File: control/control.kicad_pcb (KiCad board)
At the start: 2 copper layers, 39.1 x 45.8 mm, 37 parts, among them J1 AVR-ISP-6, J2 Conn_01x07_Pin, J3 Conn_01x02_Pin, J4 Conn_01x04_Socket, P1 Conn_01x03_Pin, P2 Conn_01x03_Pin, P3 Conn_01x03_Pin, P4 Conn_01x03_Pin, SW1 SW_Push, U2 ATmega328P-A, Y1 16MHz

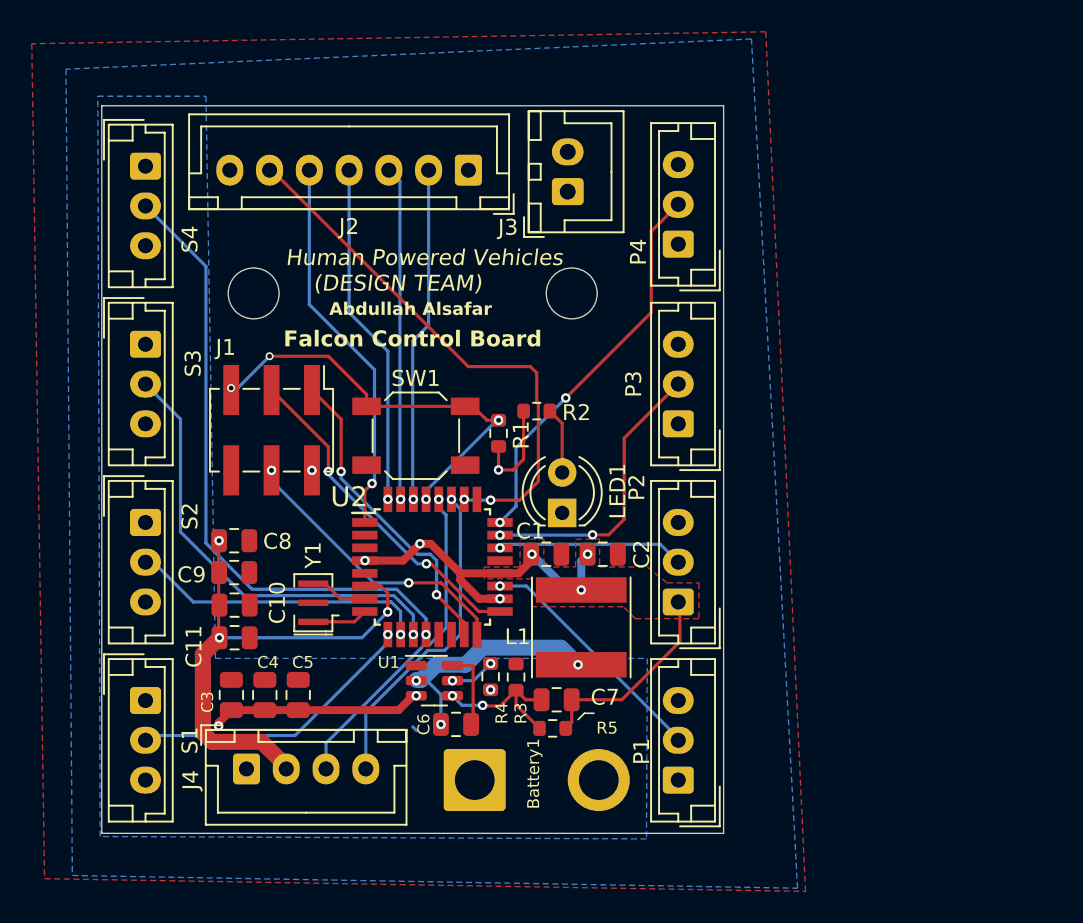
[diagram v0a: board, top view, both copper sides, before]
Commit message: Revised hardware
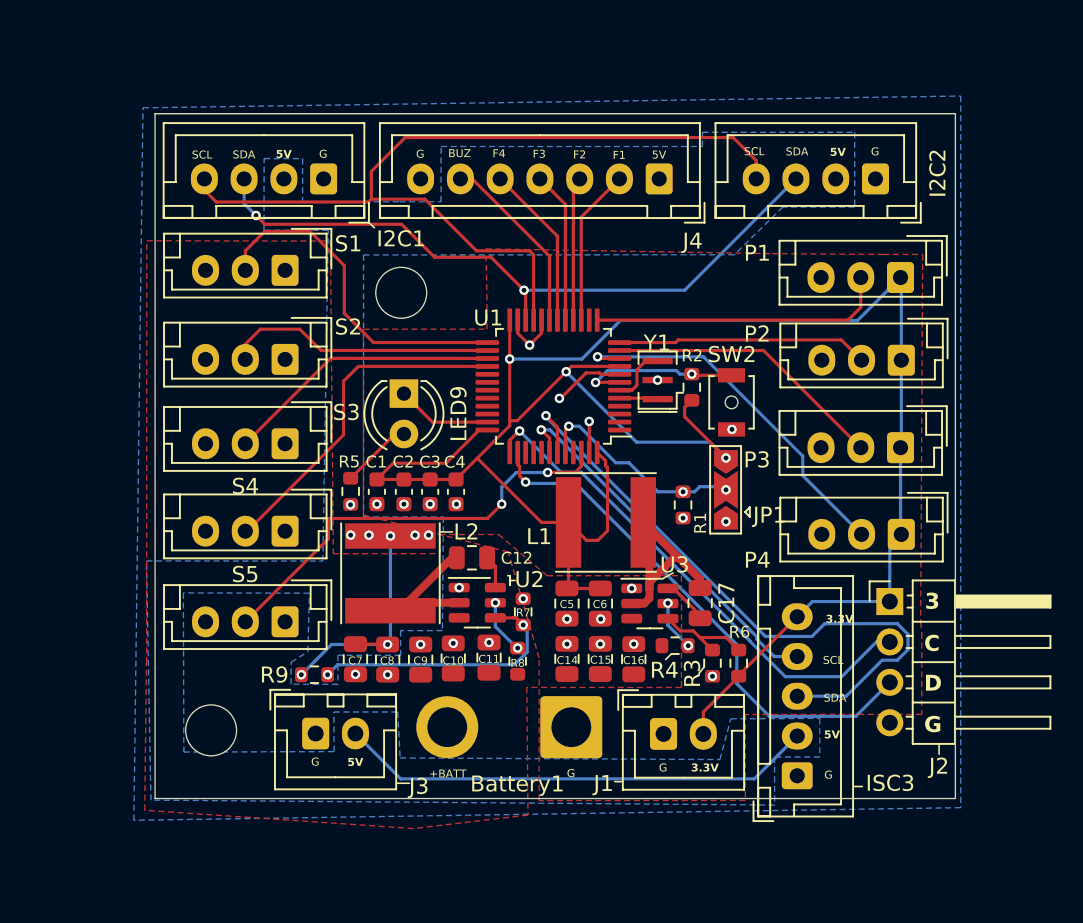
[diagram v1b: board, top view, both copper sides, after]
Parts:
- removed HOLE1, HOLE2: MountingHole_3.2mm_M3, MountingHole:MountingHole_3.2mm_M3
- removed LED1: LED1, LED_THT:LED_D4.0mm
- removed SW1: SW_Push, Button_Switch_SMD:SW_SPST_SKQG_WithoutStem
- added C12: 0.1uF, Capacitor_SMD:C_0805_2012Metric, F.Cu at (135.7, 84.4)
- added C14: 22uF, Capacitor_SMD:C_0805_2012Metric, F.Cu at (141.7, 90.8)
- added C15: 22uF, Capacitor_SMD:C_0805_2012Metric, F.Cu at (143.8, 90.8)
- added C16: 22uF, Capacitor_SMD:C_0805_2012Metric, F.Cu at (145.9, 90.8)
- added C17: 0.1uF, Capacitor_SMD:C_0805_2012Metric, F.Cu at (150.1, 87.3)
- added I2C1: FS2, Connector_JST:JST_XH_B4B-XH-A_1x04_P2.50mm_Vertical, F.Cu at (126.4, 60.6)
- added I2C2: FS1, Connector_JST:JST_XH_B4B-XH-A_1x04_P2.50mm_Vertical, F.Cu at (161.1, 60.6)
- added ISC3: MAIN, Connector_JST:JST_XH_B5B-XH-A_1x05_P2.50mm_Vertical, F.Cu at (156.2, 98.1)
- added JP1: Jumper_3_Open, Jumper:SolderJumper-3_P2.0mm_Open_TrianglePad1.0x1.5mm, F.Cu at (151.7, 80.2)
- added L2: 3.3uH, Inductor_SMD:L_Taiyo-Yuden_NR-60xx, F.Cu at (130.6, 85.4)
- added LED9: LED1, LED_THT:LED_D4.0mm, F.Cu at (131.4, 74.1)
- added R6: 33.2k, Resistor_SMD:R_0603_1608Metric, F.Cu at (152.5, 91.0)
- added R7: 10k, Resistor_SMD:R_0603_1608Metric, F.Cu at (138.9, 87.8)
- added R8: 10k, Resistor_SMD:R_0603_1608Metric, F.Cu at (138.6, 90.9)
- added R9: 54.9k, Resistor_SMD:R_0603_1608Metric, F.Cu at (125.8, 91.8)
- added REF**: MountingHole_3.2mm_M3, MountingHole:MountingHole_3.2mm_M3, F.Cu at (119.3, 95.3)
- added REF**: MountingHole_3.2mm_M3, MountingHole:MountingHole_3.2mm_M3, F.Cu at (131.3, 67.8)
- added S5: Conn_01x03_Pin, Connector_JST:JST_EH_B3B-EH-A_1x03_P2.50mm_Vertical, F.Cu at (124.0, 88.5)
- added SW2: SW_Push, Button_Switch_SMD:SW_SPST_B3U-1000P-B, F.Cu at (152.1, 74.7)
- added U3: ~, Package_TO_SOT_SMD:TSOT-23-6, F.Cu at (146.9, 87.3)
- C1, C2, C3, C4: value 22uF -> 100n; footprint Capacitor_SMD:C_0805_2012Metric -> Capacitor_SMD:C_0603_1608Metric
- C10, C9: value 100nF -> 22uF
- C11: value 10nF -> 22uF
- C6, C7: value 0.1uF -> 22uF
- C8: value 1uF -> 22uF
- J1: value AVR-ISP-6 -> Conn_01x02_Pin; footprint Connector_PinHeader_2.54mm:PinHeader_2x03_P2.54mm_Vertical_SMD -> Connector_JST:JST_XH_B2B-XH-A_1x02_P2.50mm_Vertical
- J2: value Conn_01x07_Pin -> Conn_01x04_Male; footprint Connector_JST:JST_XH_B7B-XH-A_1x07_P2.50mm_Vertical -> Connector_PinHeader_2.54mm:PinHeader_1x04_P2.54mm_Horizontal
- J4: value Conn_01x04_Socket -> Conn_01x07_Pin; footprint Connector_JST:JST_XH_B4B-XH-A_1x04_P2.50mm_Vertical -> Connector_JST:JST_XH_B7B-XH-A_1x07_P2.50mm_Vertical
- R2: value 420 -> 10k
- R5: value 54.9k -> 420
- U1: value ~ -> STM32F103C8Tx; footprint Package_TO_SOT_SMD:TSOT-23-6 -> Package_QFP:LQFP-48_7x7mm_P0.5mm
- U2: value ATmega328P-A -> ~; footprint Package_QFP:TQFP-32_7x7mm_P0.8mm -> Package_TO_SOT_SMD:TSOT-23-6
- Y1: value 16MHz -> 8Mhz
- moved J4 45.3 mm to (147.5, 60.6), turned to 180 degrees
- moved J2 37.9 mm to (162.0, 87.2), turned to 0 degrees
- moved J3 37.6 mm to (125.9, 95.5), turned to 0 degrees
- moved P1 34.6 mm to (162.7, 66.8), turned to 180 degrees
- moved J1 31.2 mm to (147.8, 95.5), turned to 0 degrees
- moved S1 28.4 mm to (124.0, 66.3), turned to 180 degrees
- moved Y1 25.8 mm to (147.4, 73.2)
- moved S4 24.6 mm to (124.0, 82.8), turned to 180 degrees
- moved P4 23.0 mm to (162.7, 83.0), turned to 180 degrees
- moved P2 20.7 mm to (162.7, 72.0), turned to 180 degrees
- moved U1 20.0 mm to (140.9, 73.6), turned to 180 degrees
- moved R5 19.6 mm to (128.1, 80.2), turned to -90 degrees
- moved C3 17.9 mm to (133.1, 80.3)
- moved C5 17.9 mm to (141.7, 87.3)
- moved C4 17.5 mm to (134.7, 80.3), turned to -90 degrees
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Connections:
- C1 pad 2: +5V -> +3.3V
- C10 pad 1: +5V -> +BATT
- C11 pad 1: +5V -> +BATT
- C2 pad 2: +5V -> +3.3V
- C3 pad 1: +BATT -> GND
- C3 pad 2: GND -> +3.3V
- C4 pad 1: +BATT -> +3.3V
- C5 pad 1: +BATT -> GND
- C5 pad 2: GND -> +3.3V
- C6 pad 1: Net-(U1-SW) -> GND
- C6 pad 2: Net-(U1-VBST) -> +3.3V
- C7 pad 1: Net-(U1-VFB) -> GND
- C8 pad 1: +5V -> GND
- C8 pad 2: GND -> +5V
- C9 pad 1: +5V -> +BATT
- J1 pad 1: MISO -> GND
- J1 pad 2: +5V -> +3.3V
- J2 pad 1: +5V -> +3.3V
- J2 pad 2: LED_{FIELD1} -> SWCLK
- J2 pad 3: LED_{FIELD2} -> SWDIO
- J2 pad 4: LED_{FIELD3} -> GND
- J4 pad 1: GND -> +5V
- J4 pad 2: +5V -> LED_{FIELD1}
- J4 pad 3: SDA -> LED_{FIELD2}
- J4 pad 4: SCL -> LED_{FIELD3}
- L1 pad 1: +5V -> +3.3V
- L1 pad 2: Net-(U1-SW) -> Net-(U3-SW)
- P1 pad 1: +5V -> +3.3V
- P2 pad 1: +5V -> +3.3V
- P3 pad 1: +5V -> +3.3V
- P4 pad 1: +5V -> +3.3V
- R1 pad 1: RESET -> GND
- R1 pad 2: +5V -> Net-(JP1-C)
- R2 pad 1: Net-(LED1-A) -> +3.3V
- R2 pad 2: +5V -> Net-(U1-NRST)
- R3 pad 2: Net-(U1-VFB) -> Net-(U3-VFB)
- R4 pad 1: Net-(U1-EN) -> Net-(U3-EN)
- R5 pad 1: +5V -> Net-(LED9-A)
- R5 pad 2: Net-(U1-VFB) -> +5V
- U1 pad 1: GND -> unconnected-(U1-VBAT-Pad1)
- U1 pad 2: Net-(U1-SW) -> unconnected-(U1-PC13-Pad2)
- U1 pad 3: +BATT -> unconnected-(U1-PC14-Pad3)
- U1 pad 4: Net-(U1-VFB) -> unconnected-(U1-PC15-Pad4)
- U1 pad 5: Net-(U1-EN) -> Net-(U1-PD0)
- U1 pad 6: Net-(U1-VBST) -> Net-(U1-PD1)
- U2 pad 1: LED_{FIELD4} -> GND
- U2 pad 2: unconnected-(U2-PD4-Pad2) -> Net-(U2-SW)
- U2 pad 3: GND -> +BATT
- U2 pad 4: +5V -> Net-(U2-VFB)
- U2 pad 5: GND -> Net-(U2-EN)
- U2 pad 6: +5V -> Net-(U2-VBST)
- Y1 pad 1: Net-(U2-XTAL2/PB7) -> Net-(U1-PD0)
- Y1 pad 3: Net-(U2-XTAL1/PB6) -> Net-(U1-PD1)
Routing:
- net +3.3V: track 0.00 -> 135.6 mm, vias 0 -> 3
- net SCL_{TOCTRL}: track 0.00 -> 55.9 mm
- net SDA_{TOCTRL}: track 0.00 -> 43.3 mm, vias 0 -> 2
- net SDA_{TOMAIN}: track 0.00 -> 41.0 mm, vias 0 -> 1
- net +5V: track 82.1 -> 45.2 mm, vias 11 -> 8
- net SWDIO: track 0.00 -> 33.4 mm, vias 0 -> 1
- net SWCLK: track 0.00 -> 32.2 mm, vias 0 -> 1
- net SER5: track 0.00 -> 27.4 mm, vias 0 -> 2
- net RESET: track 26.8 -> 0.00 mm, vias 4 -> 0
- net SCL_{TOMAIN}: track 0.00 -> 23.7 mm, vias 0 -> 1
- net BUZ: track 34.1 -> 11.6 mm, vias 2 -> 0
- net SCK: track 21.2 -> 0.00 mm, vias 2 -> 0
- net SDA: track 20.4 -> 0.00 mm, vias 1 -> 0
- net SCL: track 20.3 -> 0.00 mm, vias 1 -> 0
- net MISO: track 19.8 -> 0.00 mm, vias 2 -> 0
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- added copper zone on F.Cu, net +3.3V
- added copper zone on F.Cu, net +BATT
- added copper zone on B.Cu, net GND
- removed copper zone on F.Cu, net +5V
- removed copper zone on B.Cu, net +BATT
- removed copper zone on F.Cu, net GND
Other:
- board size 39.1 x 45.8 mm -> 50.3 x 43.1 mm
- board text added: "+BATT"
- board text added: "3"
- board text added: "3.3V"
- board text added: "5V"
- board text added: "BUZ"
- board text added: "C"
- board text added: "D"
- board text added: "F1"
- board text added: "F2"
- board text added: "F3"
- board text added: "F4"
- board text added: "G"
- board text added: "SCL"
- board text added: "SDA"
- board text removed: "Abdullah Alsafar"
- board text removed: "Distance between the center of the 2 mounting holes is 18.4532mm X: 18.4000mm Y: 1.4000mm"
- board text removed: "Distance from top-left corner to bottom-right corner: 60.1820mm X: 39.1000mm Y: 45.7500mm"
- board text removed: "Falcon Control Board"
- board text removed: "Human Powered Vehicles (DESIGN TEAM)"
